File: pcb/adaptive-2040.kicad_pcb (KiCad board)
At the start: 2 copper layers, 54.4 x 80.8 mm, 24 parts, among them J1 USB_A, J10 AudioJack2, J11 AudioJack2, J12 AudioJack2, J13 AudioJack2, J14 AudioJack2, J15 AudioJack2, J16 AudioJack2, J17 AudioJack2, J18 AudioJack2, J19 AudioJack2, J2 AudioJack2, J3 AudioJack2, J4 AudioJack2, J5 AudioJack2, J6 AudioJack2, J7 AudioJack2, J8 AudioJack2, J9 AudioJack2, U1 RaspberryPi_Pico

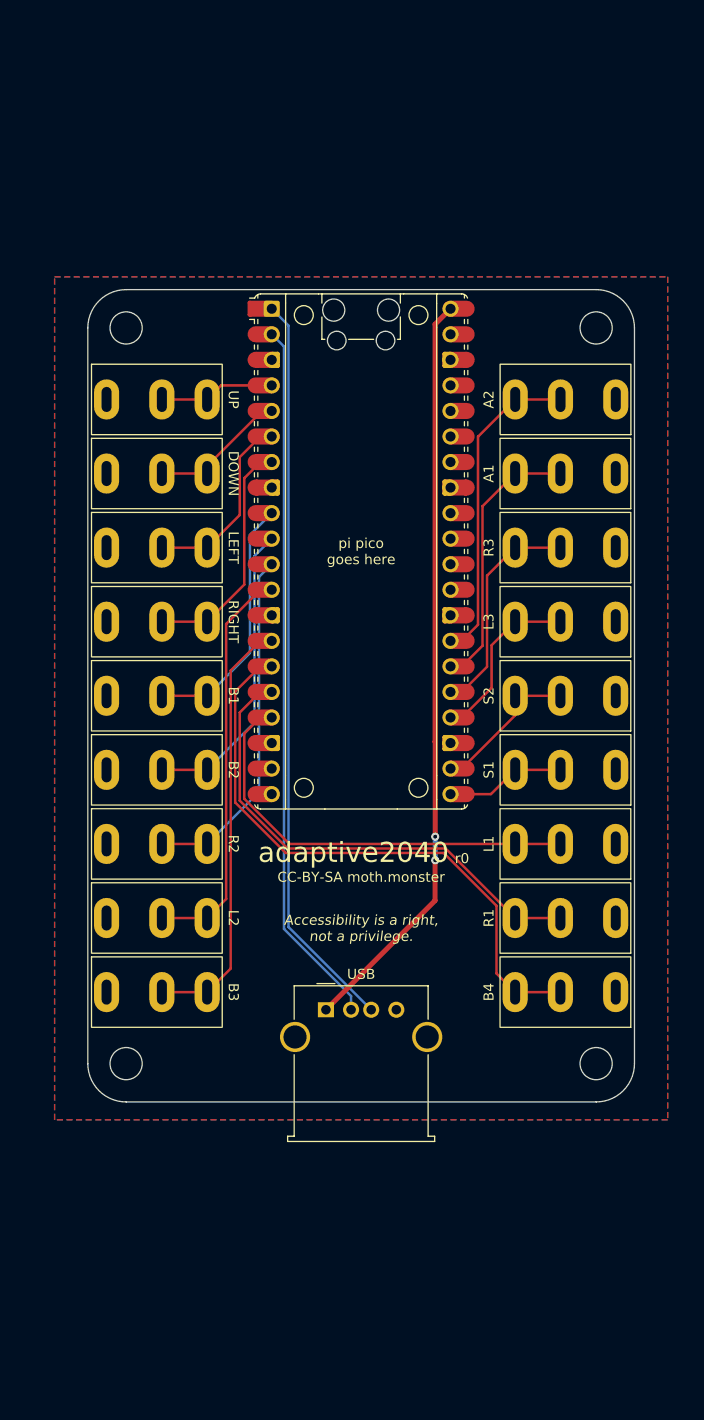
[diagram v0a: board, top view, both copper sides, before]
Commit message: r1 board
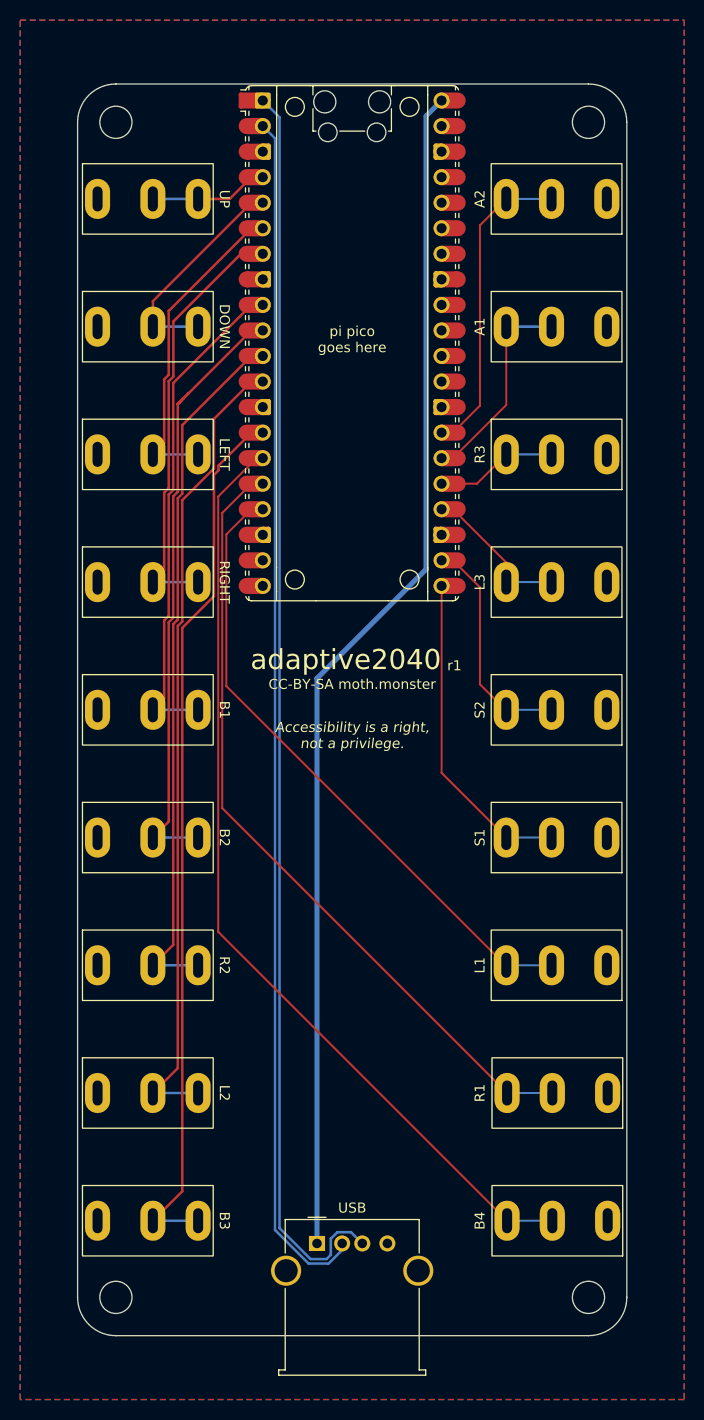
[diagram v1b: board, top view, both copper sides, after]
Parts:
- moved REF13 23.3 mm to (80.6, 208.3)
- moved J1 23.3 mm to (100.6, 202.9)
- moved REF14145235 23.3 mm to (127.6, 208.3)
- moved J10 22.8 mm to (83.8, 200.7)
- moved J11 22.7 mm to (124.5, 200.7)
- moved U1 20.7 mm to (104.1, 113.4)
- moved REF11 20.5 mm to (80.6, 91.4)
- moved REF12 20.5 mm to (127.6, 91.4)
- moved J2 20.0 mm to (83.8, 99.1)
- moved J19 20.0 mm to (124.5, 99.1)
- moved J9 17.4 mm to (83.8, 188.0)
- moved J12 17.4 mm to (124.5, 188.0)
- moved J3 14.6 mm to (83.8, 111.8)
- moved J18 14.6 mm to (124.5, 111.8)
- moved J8 12.1 mm to (83.8, 175.3)
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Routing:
- net DP: track 73.8 -> 124.8 mm
- net DM: track 70.4 -> 119.5 mm
- net B3: track 42.7 -> 88.1 mm
- net VBUS: track 74.8 -> 118.8 mm, vias 2 -> 0
- net L2: track 40.5 -> 80.4 mm
- net R2: track 35.0 -> 70.3 mm
- net B4: track 59.8 -> 94.4 mm
- net B2: track 30.1 -> 62.9 mm
- net R1: track 49.5 -> 79.1 mm
- net B1: track 25.3 -> 50.0 mm
- net L1: track 43.2 -> 63.6 mm
- net S1: track 11.9 -> 32.2 mm
- net RIGHT: track 23.7 -> 42.9 mm
- net LEFT: track 18.9 -> 32.2 mm
- net R3: track 22.2 -> 12.1 mm
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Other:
- board size 54.4 x 80.8 mm -> 54.6 x 124.5 mm
- board text added: "if you want your JLCPCB order number hidden by the Pico, this is a good spot to put it"
- board text added: "r1"
- board text removed: "r0"
